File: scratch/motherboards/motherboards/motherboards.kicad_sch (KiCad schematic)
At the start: 6 parts, among them J101 Conn_01x35, J102 Conn_02x35_Counter_Clockwise, J103 Conn_01x35, J104 Conn_01x35, J105 Conn_02x35_Counter_Clockwise, J106 Conn_01x35

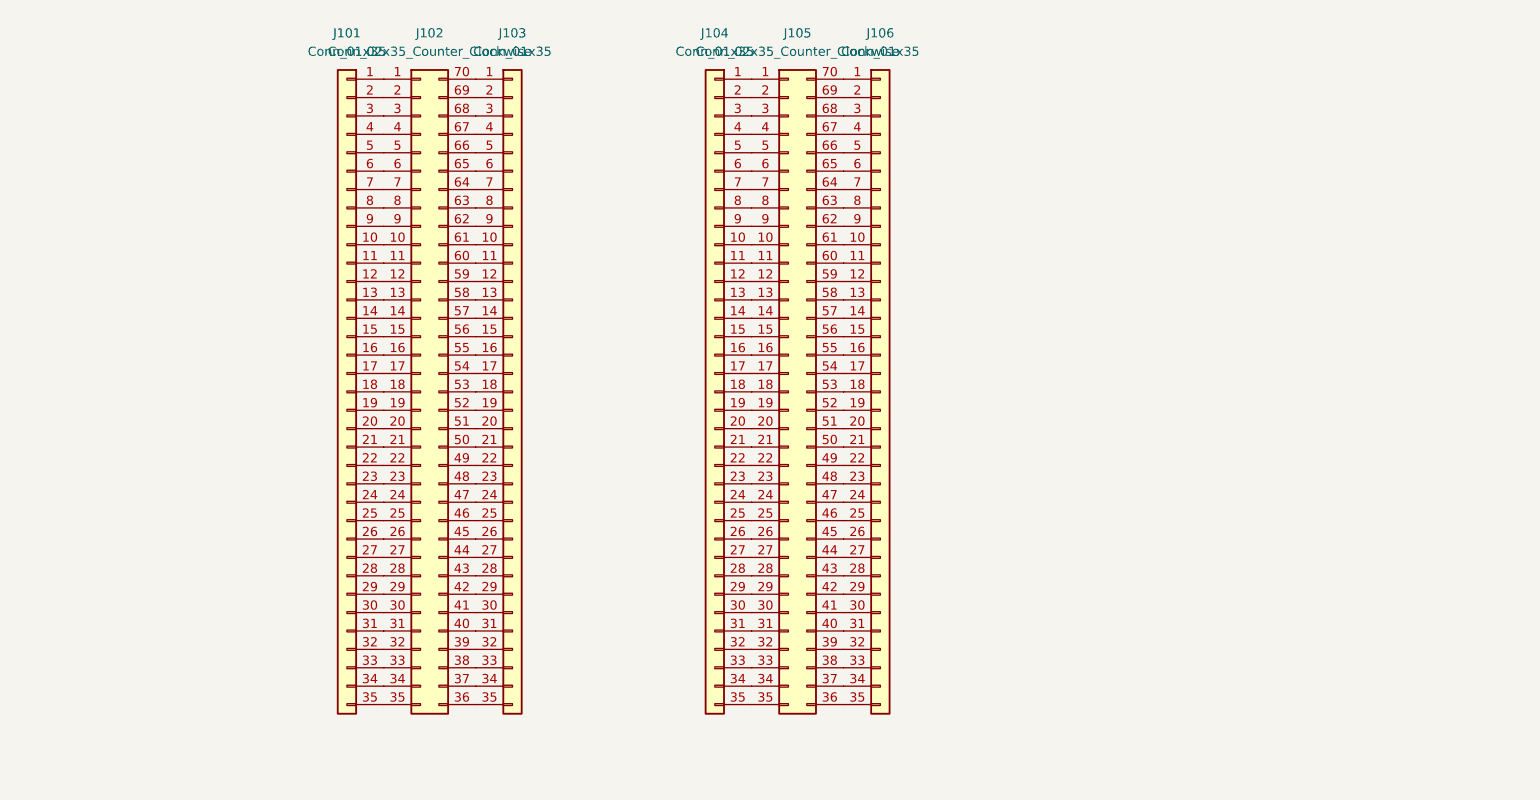
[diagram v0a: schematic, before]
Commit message: housekeeping
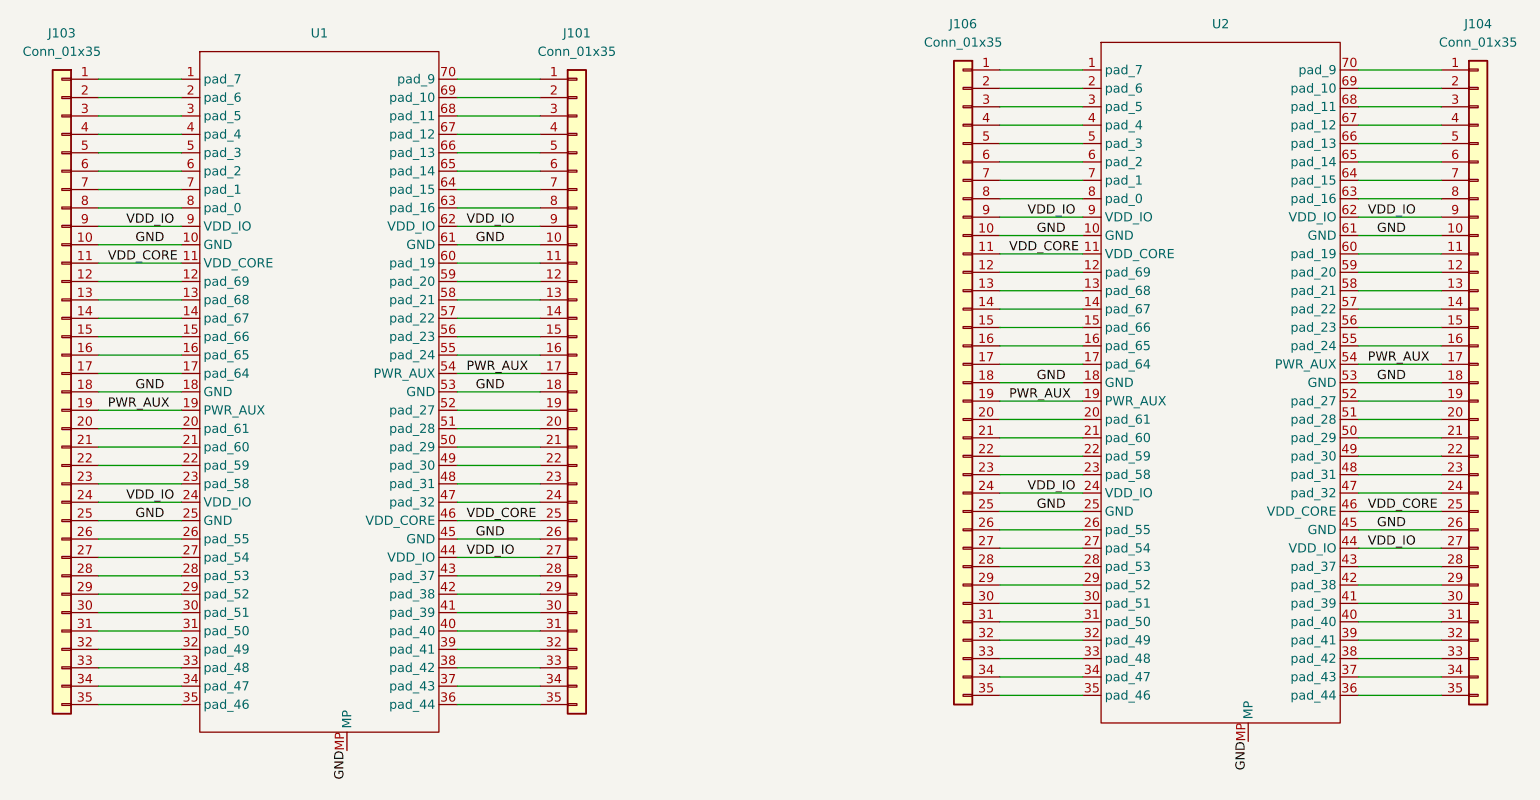
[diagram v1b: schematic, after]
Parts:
- removed J102, J105: Conn_02x35_Counter_Clockwise, Connector_Mezzanine:CONN-SMD_70P-P0.40_HC-PBB40C-70DS-0.4V-3.0-02, symbol Connector_Generic:Conn_02x35_Counter_Clockwise
- added U1, U2: ~, WaferSpace:P0.40_HC-PBB40C-70DS-0.4V-3.0-02_wscob, symbol WaferSpace:70pin_ws_default_mezzanine
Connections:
- net at J101.1 (Pin_1): now also U1.70 (pad_9)
- net GND: now reaches J101.10 (Pin_10)
- net GND: now also J101.18 (Pin_18), J101.26 (Pin_26), J103.10 (Pin_10), J103.18 (Pin_18), J103.25 (Pin_25), J104.10 (Pin_10), J104.18 (Pin_18), J104.26 (Pin_26), J106.10 (Pin_10), J106.18 (Pin_18), J106.25 (Pin_25), U1.10 (GND), U1.18 (GND), U1.25 (GND), U1.45 (GND), U1.53 (GND), U1.61 (GND), U1.MP, U2.10 (GND), U2.18 (GND), U2.25 (GND), U2.45 (GND), U2.53 (GND), U2.61 (GND), U2.MP
- net at J101.11 (Pin_11): now also U1.60 (pad_19)
- net at J101.12 (Pin_12): now also U1.59 (pad_20)
- net at J101.13 (Pin_13): now also U1.58 (pad_21)
- net at J101.14 (Pin_14): now also U1.57 (pad_22)
- net at J101.15 (Pin_15): now also U1.56 (pad_23)
- net at J101.16 (Pin_16): now also U1.55 (pad_24)
- net PWR_AUX: now reaches J101.17 (Pin_17)
- net PWR_AUX: now also J103.19 (Pin_19), J104.17 (Pin_17), J106.19 (Pin_19), U1.19 (PWR_AUX), U1.54 (PWR_AUX), U2.19 (PWR_AUX), U2.54 (PWR_AUX)
- net at J101.19 (Pin_19): now also U1.52 (pad_27)
- net at J101.2 (Pin_2): now also U1.69 (pad_10)
- net at J101.20 (Pin_20): now also U1.51 (pad_28)
- net at J101.21 (Pin_21): now also U1.50 (pad_29)
- net at J101.22 (Pin_22): now also U1.49 (pad_30)
- net at J101.23 (Pin_23): now also U1.48 (pad_31)
- net at J101.24 (Pin_24): now also U1.47 (pad_32)
- net VDD_CORE: now reaches J101.25 (Pin_25)
- net VDD_CORE: now also J103.11 (Pin_11), J104.25 (Pin_25), J106.11 (Pin_11), U1.11 (VDD_CORE), U1.46 (VDD_CORE), U2.11 (VDD_CORE), U2.46 (VDD_CORE)
- net VDD_IO: now reaches J101.27 (Pin_27)
- net VDD_IO: now also J101.9 (Pin_9), J103.24 (Pin_24), J103.9 (Pin_9), J104.27 (Pin_27), J104.9 (Pin_9), J106.24 (Pin_24), J106.9 (Pin_9), U1.24 (VDD_IO), U1.44 (VDD_IO), U1.62 (VDD_IO), U1.9 (VDD_IO), U2.24 (VDD_IO), U2.44 (VDD_IO), U2.62 (VDD_IO), U2.9 (VDD_IO)
- net at J101.28 (Pin_28): now also U1.43 (pad_37)
- net at J101.29 (Pin_29): now also U1.42 (pad_38)
- net at J101.3 (Pin_3): now also U1.68 (pad_11)
- net at J101.30 (Pin_30): now also U1.41 (pad_39)
- net at J101.31 (Pin_31): now also U1.40 (pad_40)
- net at J101.32 (Pin_32): now also U1.39 (pad_41)
- net at J101.33 (Pin_33): now also U1.38 (pad_42)
- net at J101.34 (Pin_34): now also U1.37 (pad_43)
- net at J101.35 (Pin_35): now also U1.36 (pad_44)
- net at J103.35 (Pin_35): now also U1.35 (pad_46)
- net at J103.34 (Pin_34): now also U1.34 (pad_47)
- net at J103.33 (Pin_33): now also U1.33 (pad_48)
- net at J103.32 (Pin_32): now also U1.32 (pad_49)
- net at J101.4 (Pin_4): now also U1.67 (pad_12)
- net at J103.31 (Pin_31): now also U1.31 (pad_50)
- net at J103.30 (Pin_30): now also U1.30 (pad_51)
- net at J103.29 (Pin_29): now also U1.29 (pad_52)
- net at J103.28 (Pin_28): now also U1.28 (pad_53)
- net at J103.27 (Pin_27): now also U1.27 (pad_54)
- net at J103.26 (Pin_26): now also U1.26 (pad_55)
- net at J103.23 (Pin_23): now also U1.23 (pad_58)
- net at J103.22 (Pin_22): now also U1.22 (pad_59)
- net at J101.5 (Pin_5): now also U1.66 (pad_13)
- net at J103.21 (Pin_21): now also U1.21 (pad_60)
- net at J103.20 (Pin_20): now also U1.20 (pad_61)
- net at J103.17 (Pin_17): now also U1.17 (pad_64)
- net at J103.16 (Pin_16): now also U1.16 (pad_65)
- net at J103.15 (Pin_15): now also U1.15 (pad_66)
- net at J103.14 (Pin_14): now also U1.14 (pad_67)
- net at J103.13 (Pin_13): now also U1.13 (pad_68)
- net at J103.12 (Pin_12): now also U1.12 (pad_69)
- net at J101.6 (Pin_6): now also U1.65 (pad_14)
- net at J103.8 (Pin_8): now also U1.8 (pad_0)
- net at J103.7 (Pin_7): now also U1.7 (pad_1)
- net at J103.6 (Pin_6): now also U1.6 (pad_2)
- net at J103.5 (Pin_5): now also U1.5 (pad_3)
- net at J103.4 (Pin_4): now also U1.4 (pad_4)
- net at J103.3 (Pin_3): now also U1.3 (pad_5)
- net at J103.2 (Pin_2): now also U1.2 (pad_6)
- net at J101.7 (Pin_7): now also U1.64 (pad_15)
- net at J103.1 (Pin_1): now also U1.1 (pad_7)
- net at J101.8 (Pin_8): now also U1.63 (pad_16)
- net at J106.1 (Pin_1): now also U2.1 (pad_7)
- net at J106.12 (Pin_12): now also U2.12 (pad_69)
- net at J106.13 (Pin_13): now also U2.13 (pad_68)
- net at J106.14 (Pin_14): now also U2.14 (pad_67)
- net at J106.15 (Pin_15): now also U2.15 (pad_66)
- net at J106.16 (Pin_16): now also U2.16 (pad_65)
- net at J106.17 (Pin_17): now also U2.17 (pad_64)
- net at J106.2 (Pin_2): now also U2.2 (pad_6)
- net at J106.20 (Pin_20): now also U2.20 (pad_61)
- net at J106.21 (Pin_21): now also U2.21 (pad_60)
- net at J106.22 (Pin_22): now also U2.22 (pad_59)
- net at J106.23 (Pin_23): now also U2.23 (pad_58)
- net at J106.26 (Pin_26): now also U2.26 (pad_55)
- net at J106.27 (Pin_27): now also U2.27 (pad_54)
- net at J106.28 (Pin_28): now also U2.28 (pad_53)
- net at J106.29 (Pin_29): now also U2.29 (pad_52)
- net at J106.3 (Pin_3): now also U2.3 (pad_5)
- net at J106.30 (Pin_30): now also U2.30 (pad_51)
- net at J106.31 (Pin_31): now also U2.31 (pad_50)
- net at J106.32 (Pin_32): now also U2.32 (pad_49)
- net at J106.33 (Pin_33): now also U2.33 (pad_48)
- net at J106.34 (Pin_34): now also U2.34 (pad_47)
- net at J106.35 (Pin_35): now also U2.35 (pad_46)
- net at J106.4 (Pin_4): now also U2.4 (pad_4)
- net at J106.5 (Pin_5): now also U2.5 (pad_3)
- net at J106.6 (Pin_6): now also U2.6 (pad_2)
- net at J106.7 (Pin_7): now also U2.7 (pad_1)
- net at J106.8 (Pin_8): now also U2.8 (pad_0)
- net at J104.1 (Pin_1): now also U2.70 (pad_9)
- net at J104.11 (Pin_11): now also U2.60 (pad_19)
- net at J104.12 (Pin_12): now also U2.59 (pad_20)
- net at J104.13 (Pin_13): now also U2.58 (pad_21)
- net at J104.14 (Pin_14): now also U2.57 (pad_22)
- net at J104.15 (Pin_15): now also U2.56 (pad_23)
- net at J104.16 (Pin_16): now also U2.55 (pad_24)
- net at J104.19 (Pin_19): now also U2.52 (pad_27)
- net at J104.2 (Pin_2): now also U2.69 (pad_10)
- net at J104.20 (Pin_20): now also U2.51 (pad_28)
- net at J104.21 (Pin_21): now also U2.50 (pad_29)
- net at J104.22 (Pin_22): now also U2.49 (pad_30)
- net at J104.23 (Pin_23): now also U2.48 (pad_31)
- net at J104.24 (Pin_24): now also U2.47 (pad_32)
- net at J104.28 (Pin_28): now also U2.43 (pad_37)
- net at J104.29 (Pin_29): now also U2.42 (pad_38)
- net at J104.3 (Pin_3): now also U2.68 (pad_11)
- net at J104.30 (Pin_30): now also U2.41 (pad_39)
- net at J104.31 (Pin_31): now also U2.40 (pad_40)
- net at J104.32 (Pin_32): now also U2.39 (pad_41)
- net at J104.33 (Pin_33): now also U2.38 (pad_42)
- net at J104.34 (Pin_34): now also U2.37 (pad_43)
- net at J104.35 (Pin_35): now also U2.36 (pad_44)
- net at J104.4 (Pin_4): now also U2.67 (pad_12)
- net at J104.5 (Pin_5): now also U2.66 (pad_13)
- net at J104.6 (Pin_6): now also U2.65 (pad_14)
- net at J104.7 (Pin_7): now also U2.64 (pad_15)
- net at J104.8 (Pin_8): now also U2.63 (pad_16)
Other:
- moved on the sheet: J101, J103, J104, J106
